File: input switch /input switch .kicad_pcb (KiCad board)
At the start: 2 copper layers, 10 parts, among them IC1 MCP23008T-E_SS, IC2 ULN2003ADR, J1 BHR-06-VUA, J2 825433-8, U1 TLP293-4, U2 TLP293-4

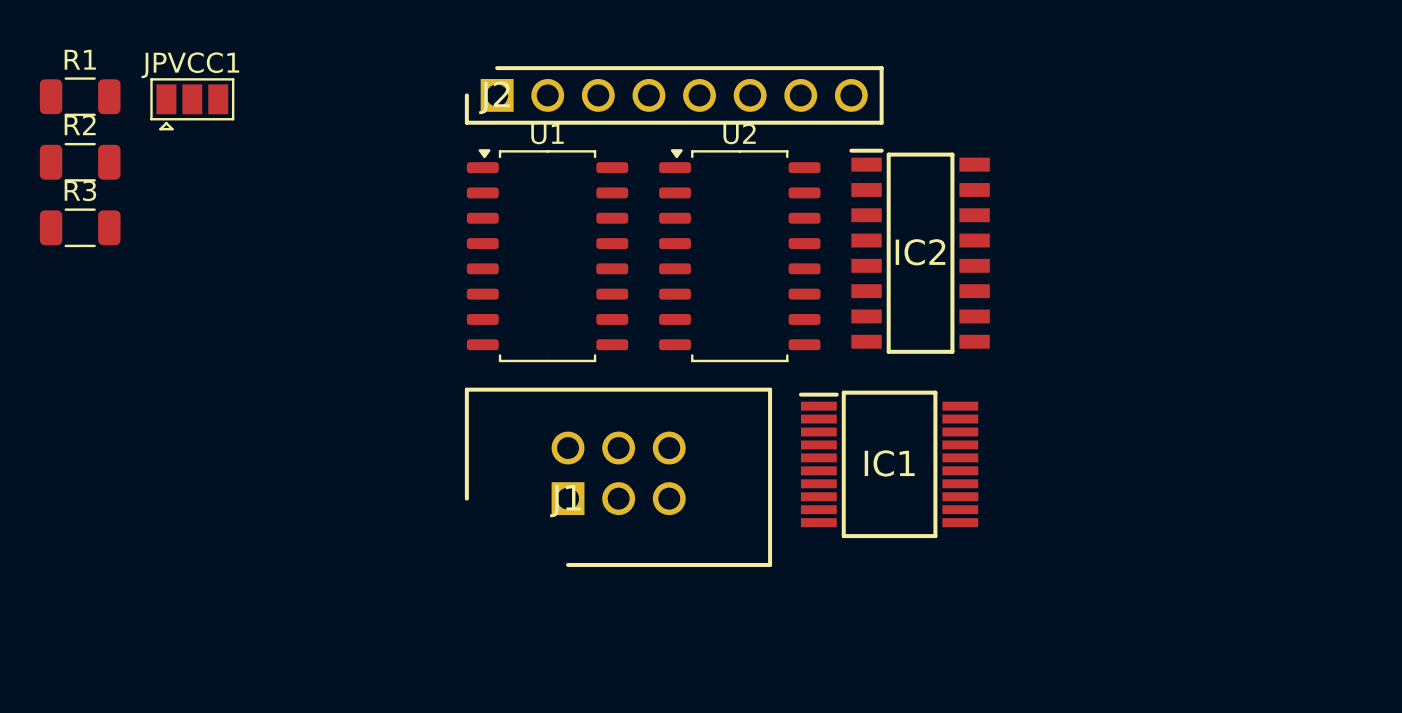
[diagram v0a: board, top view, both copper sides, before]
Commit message: likely all done with v1, mainboard obsolete
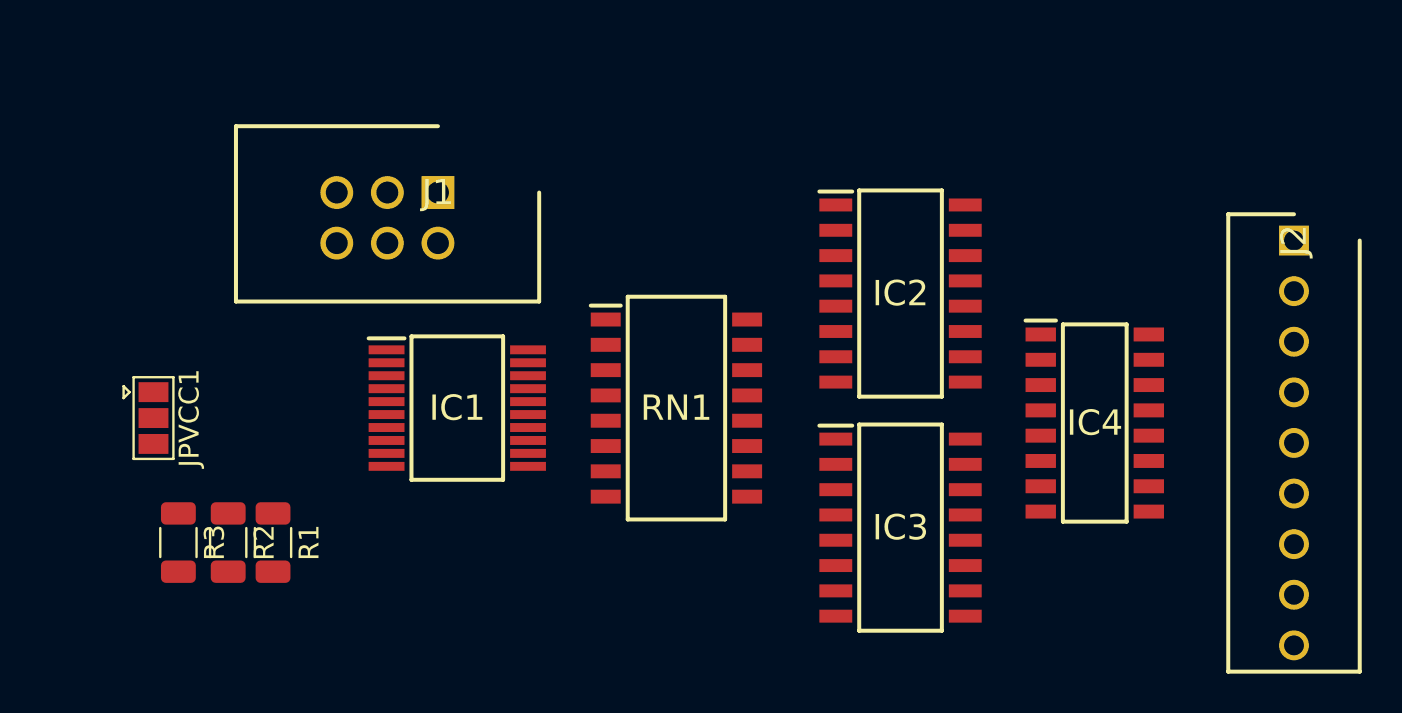
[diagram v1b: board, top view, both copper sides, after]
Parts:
- removed U1, U2: TLP293-4, Package_SO:SOIC-16_4.55x10.3mm_P1.27mm
- added IC3: TLP293-4_GB,E, Samacsys:SOIC127P700X220-16N, F.Cu at (145.2, 102.0)
- added IC4: ULN2003ADR, Samacsys:SOIC127P600X175-16N, F.Cu at (155.0, 96.8)
- added RN1: 4816P-1-221LF, Samacsys:SOIC127P762X240-16N, F.Cu at (134.0, 96.0)
- IC2: value ULN2003ADR -> TLP293-4_GB,E; footprint Samacsys:SOIC127P600X175-16N -> Samacsys:SOIC127P700X220-16N
- J2: value 825433-8 -> 22-23-2091; footprint Samacsys:HDRV8W63P0X254_1X8_2032X254X970P -> Samacsys:HDRV9W82P0X254_1X9_2271X635X1066P
- moved J2 40.7 mm to (165.0, 87.6), turned to -90 degrees
- moved R3 22.9 mm to (109.0, 102.8), turned to -90 degrees
- moved IC1 21.9 mm to (123.0, 96.0)
- moved R1 21.4 mm to (113.8, 102.8), turned to -90 degrees
- moved R2 17.5 mm to (111.5, 102.8), turned to -90 degrees
- moved J1 16.7 mm to (122.0, 85.2), turned to 180 degrees
- moved JPVCC1 16.1 mm to (107.8, 96.5), turned to -90 degrees
- moved IC2 2.26 mm to (145.2, 90.2)
- renumbered R2 to R1, R3 to R2, R1 to R3
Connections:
- IC2 pad 1: Net-(IC2-1B) -> unconnected-(IC2-ANODE_1-Pad1)
- IC2 pad 10: Net-(IC2-7C) -> VCC
- IC2 pad 11: Net-(IC2-6C) -> Net-(IC2-EMITTER_2)
- IC2 pad 12: Net-(IC2-5C) -> VCC
- IC2 pad 13: Net-(IC2-4C) -> Net-(IC2-EMITTER_3)
- IC2 pad 14: Net-(IC2-3C) -> VCC
- IC2 pad 15: Net-(IC2-2C) -> unconnected-(IC2-EMITTER_4-Pad15)
- IC2 pad 16: VCC -> unconnected-(IC2-COLLECTOR_4-Pad16)
- IC2 pad 2: Net-(IC2-2B) -> unconnected-(IC2-CATHODE_1-Pad2)
- IC2 pad 4: Net-(IC2-4B) -> GNDD
- IC2 pad 6: Net-(IC2-6B) -> GNDD
- IC2 pad 8: Net-(IC2-E) -> GNDD
- IC2 pad 9: VCC -> Net-(IC2-EMITTER_1)
- J2 pad 1: Net-(IC2-E) -> VCC
- J2 pad 2: VCC -> Net-(IC4-E)
- J2 pad 3: Net-(IC2-2C) -> Net-(IC4-1C)
- J2 pad 4: Net-(IC2-3C) -> Net-(IC4-2C)
- J2 pad 5: Net-(IC2-4C) -> Net-(IC4-3C)
- J2 pad 6: Net-(IC2-5C) -> Net-(IC4-4C)
- J2 pad 7: Net-(IC2-6C) -> Net-(IC4-5C)
- J2 pad 8: Net-(IC2-7C) -> Net-(IC4-6C)
